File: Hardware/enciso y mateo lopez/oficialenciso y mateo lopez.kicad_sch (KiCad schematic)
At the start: 14 parts, among them K1 SANYOU_SRD_Form_C, K2 SANYOU_SRD_Form_C, K3 SANYOU_SRD_Form_C, K4 SANYOU_SRD_Form_C, Q1 BC547, U1 ESP32-WROOM-32

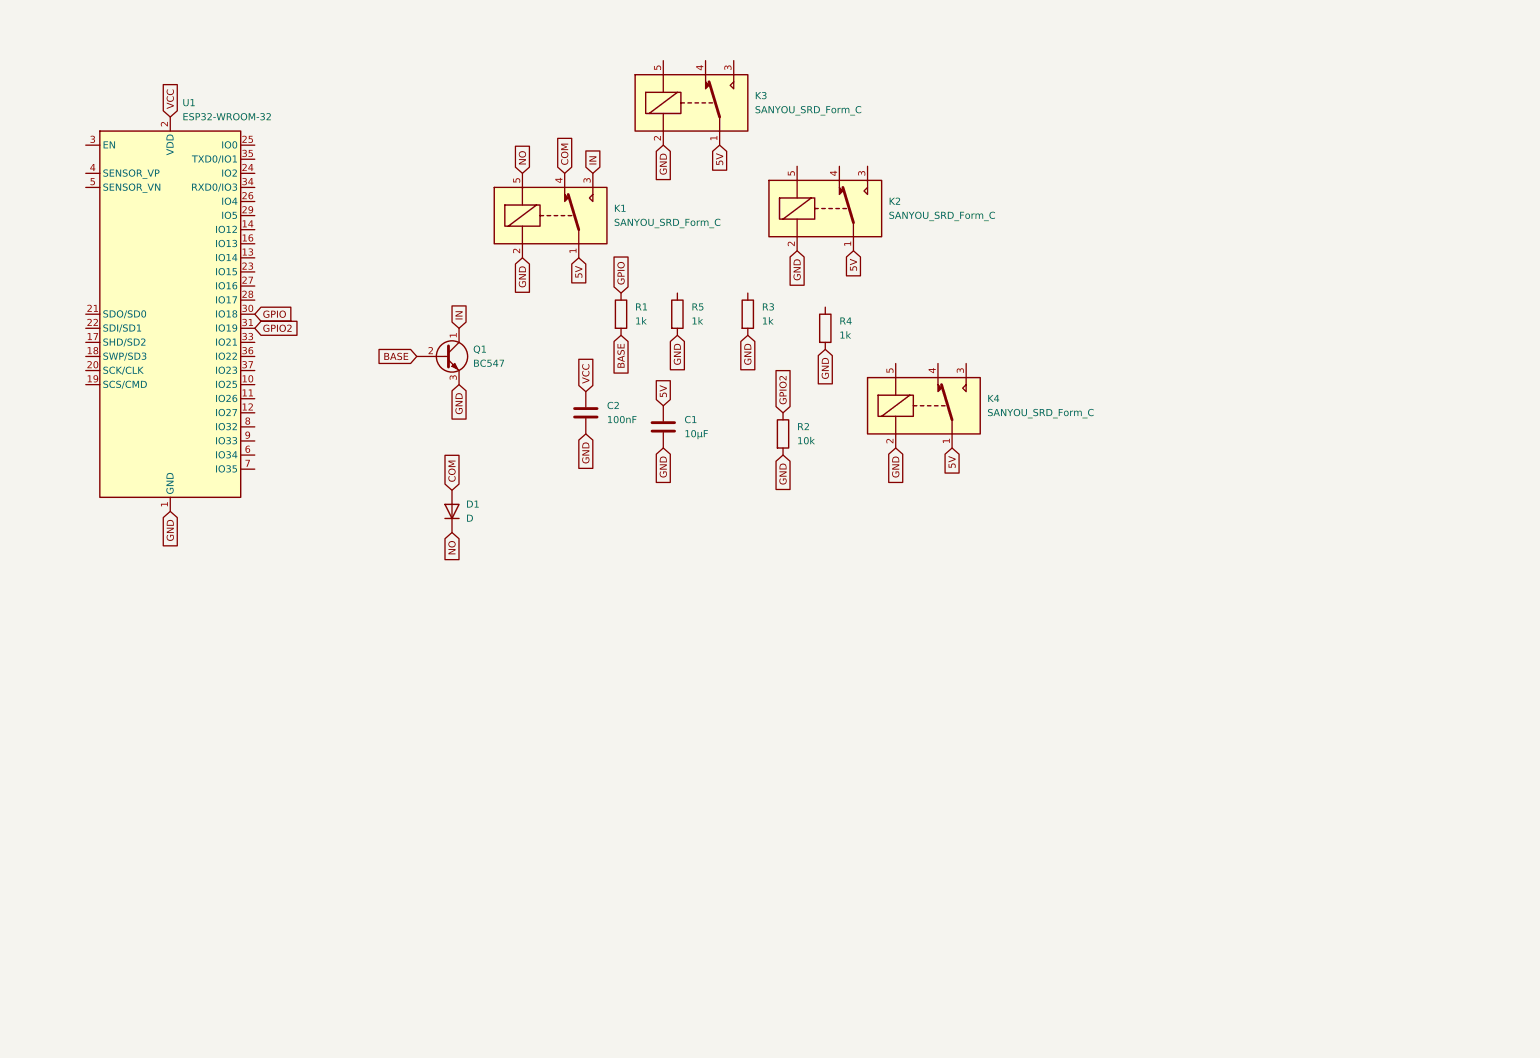
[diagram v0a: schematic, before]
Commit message: ESQUEMA GOD
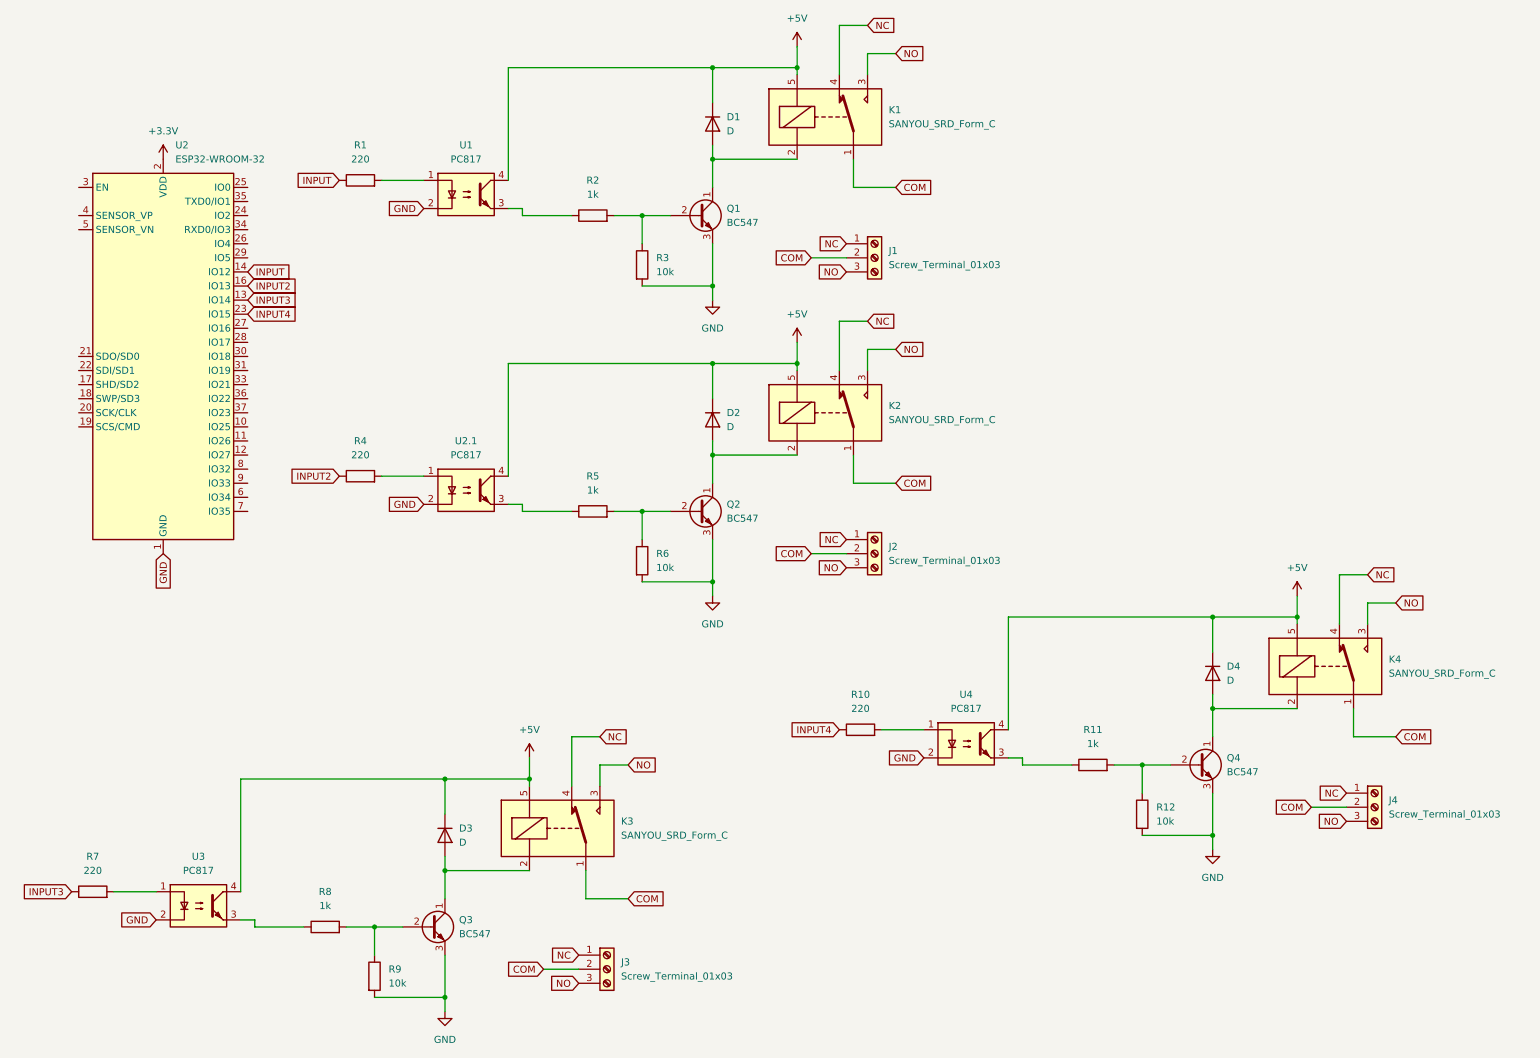
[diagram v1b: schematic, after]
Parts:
- removed C1: 10µF, Capacitor_THT:CP_Radial_D10.0mm_P5.00mm, symbol Device:C
- removed C2: 100nF, Capacitor_THT:CP_Radial_D10.0mm_P5.00mm, symbol Device:C
- removed U1: ESP32-WROOM-32, RF_Module:ESP32-WROOM-32, symbol RF_Module:ESP32-WROOM-32
- added D2, D3, D4: D, Diode_THT:D_5W_P12.70mm_Horizontal, symbol Device:D
- added J1, J2, J3, J4: Screw_Terminal_01x03, symbol Connector:Screw_Terminal_01x03
- added Q2, Q3, Q4: BC547, Package_TO_SOT_THT:TO-92_Inline, symbol Transistor_BJT:BC547
- added R10, R7: 220, Resistor_SMD:R_0805_2012Metric, symbol Device:R
- added R11, R8: 1k, Resistor_SMD:R_0805_2012Metric, symbol Device:R
- added R12, R6, R9: 10k, Resistor_SMD:R_0805_2012Metric, symbol Device:R
- added U1, U2.1, U3, U4: PC817, Package_DIP:DIP-4_W7.62mm, symbol Isolator:PC817
- added U2: ESP32-WROOM-32, RF_Module:ESP32-WROOM-32, symbol RF_Module:ESP32-WROOM-32
- R1, R4: value 1k -> 220
- R2: value 10k -> 1k
- R3: value 1k -> 10k
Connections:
- net 5V is gone; now on net COM: K1.1, K2.1, K3.1, K4.1
- net COM: now also J1.2 (Pin_2), J2.2 (Pin_2), J3.2 (Pin_2), J4.2 (Pin_2); no longer D1.2 (A), K1.4
- net GND: now also Q2.3 (E), Q3.3 (E), Q4.3 (E), R12.2, R6.2, R9.2, U1.2, U2.1 (GND), U2.1.2, U2.15 (GND), U2.38 (GND), U2.39 (GND), U3.2, U4.2; no longer K1.2, K2.2, K3.2, K4.2, R2.2, R4.2, R5.2
- net NO: now also K1.3, K2.3, K3.3, K4.3, J1.3 (Pin_3), J2.3 (Pin_3), J3.3 (Pin_3), J4.3 (Pin_3); no longer D1.1 (K), K1.5
- net NC: now reaches K2.4
- net NC: now also K1.4, K3.4, K4.4, J1.1 (Pin_1), J2.1 (Pin_1), J3.1 (Pin_1), J4.1 (Pin_1)
- net +5V: now reaches K2.5
- net +5V: now also D1.1 (K), K1.5, K3.5, K4.5, D2.1 (K), D3.1 (K), D4.1 (K), U1.4, U2.1.4, U3.4, U4.4
- net INPUT2: now reaches R4.1
- net INPUT2: now also U2.16 (IO13)
- net at R3.1: now also Q1.2 (B), R2.2
- net at R5.1: now also U2.1.3
- net BASE: no longer names the net of R1.2
- net BASE: now also U1.1; no longer Q1.2 (B)
- net GPIO renamed INPUT
- net INPUT: now also U2.14 (IO12)
- net GPIO2: no longer names the net of R2.1
- net GPIO2: now also U1.3
- net IN: no longer names the net of Q1.1 (C)
- net IN: now also D1.2 (A), K1.2; no longer K1.3
- new net: R7.2, U3.1
- new net: Q4.2 (B), R11.2, R12.1
- new net: D4.2 (A), K4.2, Q4.1 (C)
- new net: R4.2, U2.1.1
- new net: R10.2, U4.1
- new net: R11.1, U4.3
- new net: D3.2 (A), K3.2, Q3.1 (C)
- new net: Q3.2 (B), R8.2, R9.1
- new net: Q2.2 (B), R5.2, R6.1
- new net: D2.2 (A), K2.2, Q2.1 (C)
- new net: R8.1, U3.3
- new net +3.3V: U2.2 (VDD)
- new net INPUT3: R7.1, U2.13 (IO14)
- new net INPUT4: R10.1, U2.23 (IO15)
